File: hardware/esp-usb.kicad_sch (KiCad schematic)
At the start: 29 parts, among them J1 USB_A, J2 Conn_01x05, J3 Conn_01x05, J4 USB_A, SW1 SW_Push, U1 ESP32-C3, U2 SPX3819M5-L-3-3, U7 TPD2EUSB30A, Y1 Crystal_GND23

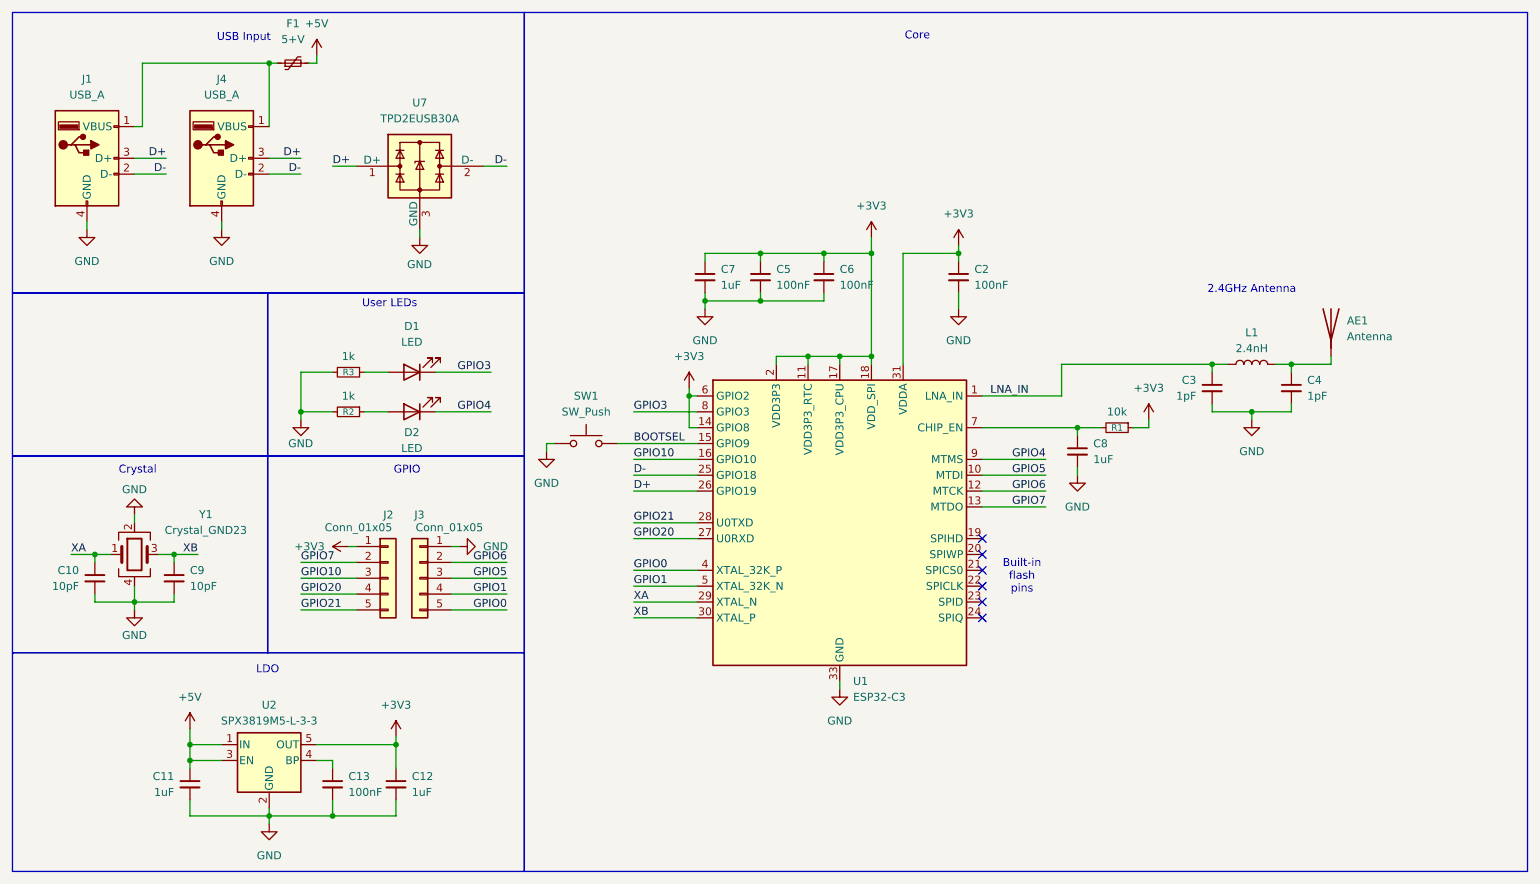
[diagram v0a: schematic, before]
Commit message: Final rev!
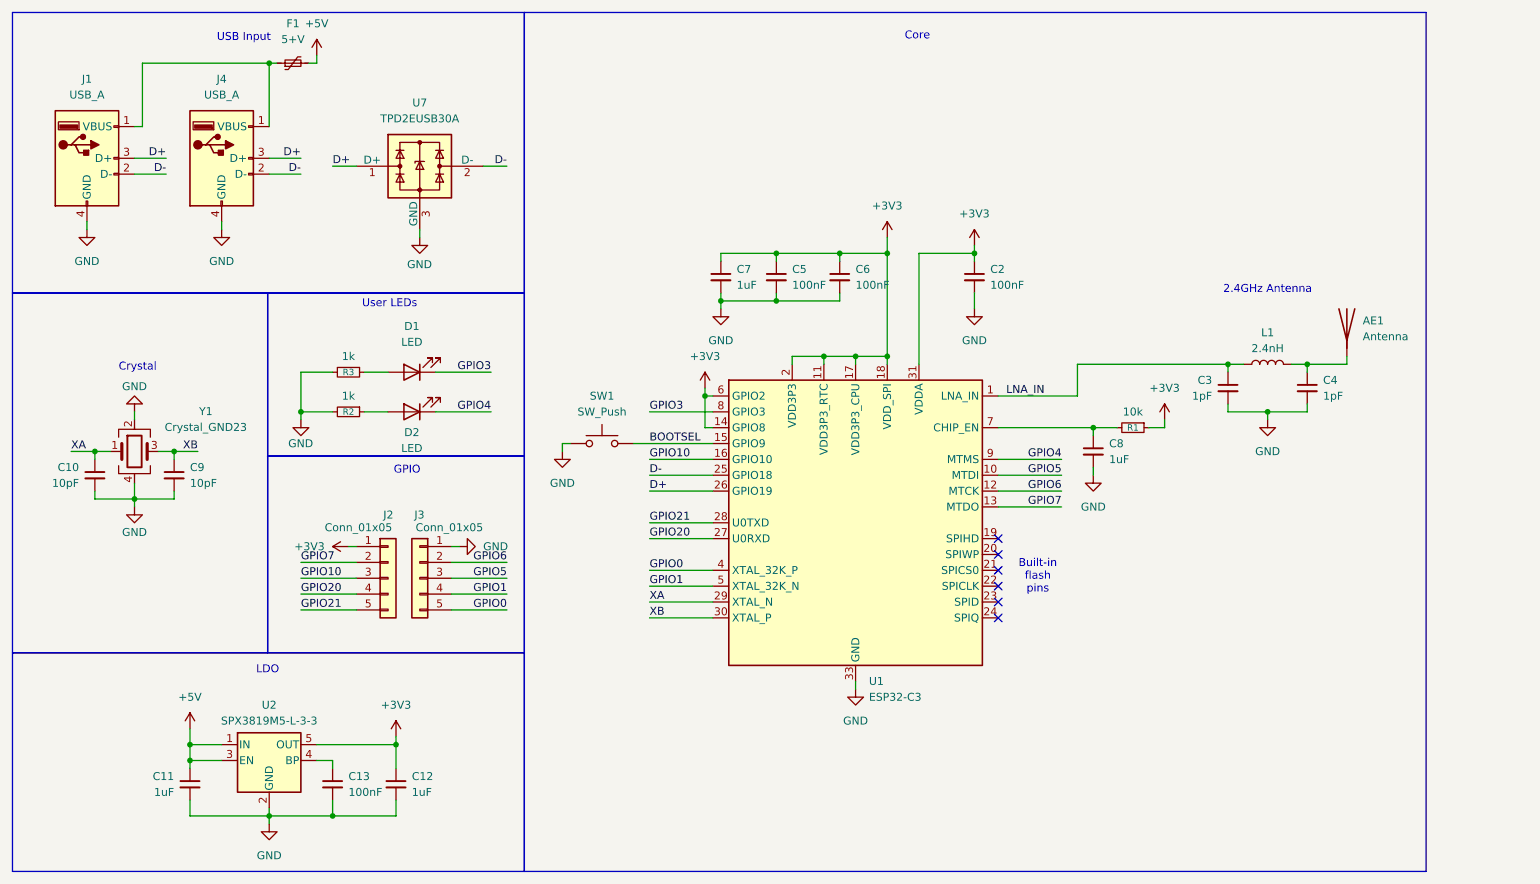
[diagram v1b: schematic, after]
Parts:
- C13, C2, C5, C6: LCSC Part # (none) -> C1525
- R1: LCSC Part # (none) -> C25744
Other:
- moved on the sheet: AE1, C10, C2, C3, C4, C5, C6, C7, C8, C9, L1, R1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
